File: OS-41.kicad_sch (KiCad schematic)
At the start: 65 parts, among them J1 Conn_02x03_Counter_Clockwise, J2 Conn_01x02_Pin, J3 Conn_01x02_Pin, J4 Conn_Coaxial, SW4 SW_Push, U1 BME280, U2 SI4432-B1-FMR, U3 MCP1640x-xCHY, U4 ATGM336H-5N31, U7 STM32F103C8Tx, Y1 32.768KHz 12.5pF, Y2 8MHz 12pF, Y3 30MHz 10pF

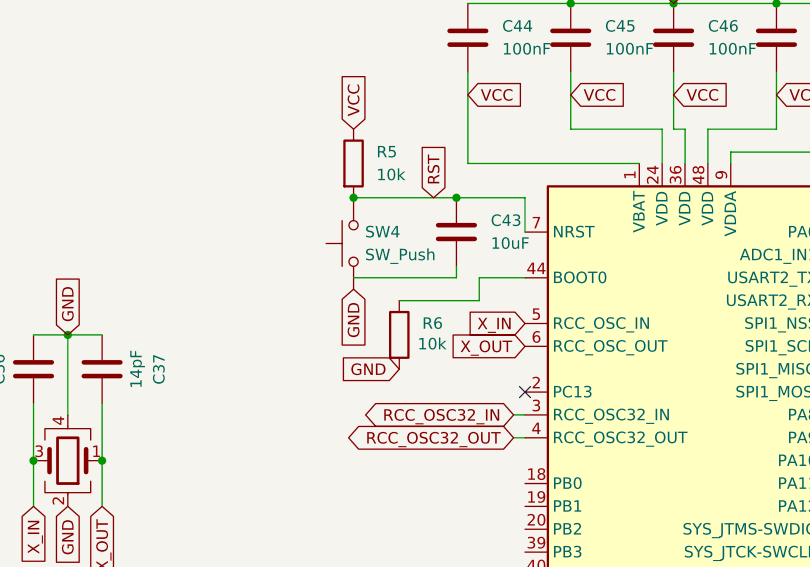
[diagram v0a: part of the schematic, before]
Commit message: Start routing!
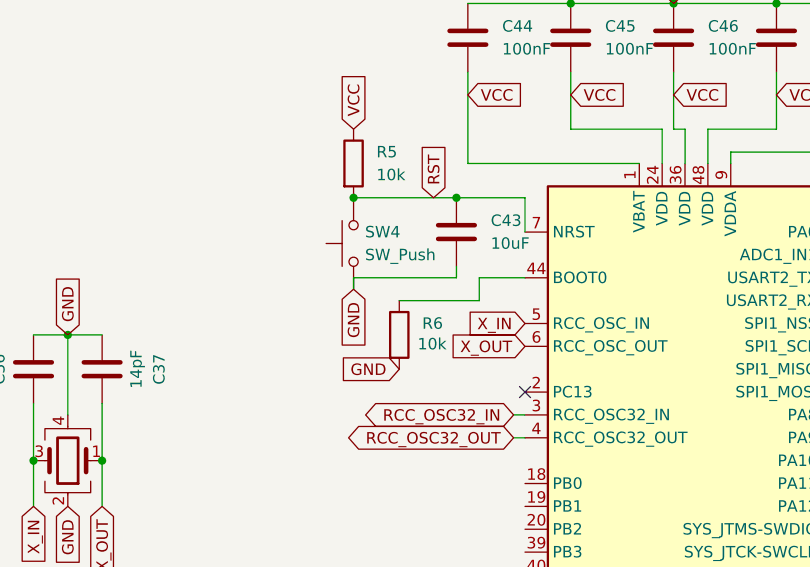
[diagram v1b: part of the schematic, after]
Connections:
- net GND: now also C43.2
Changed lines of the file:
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@@
+	(wire
+		(pts
+			(xy 283.21 60.96) (xy 271.78 60.96)
+		)
+		(stroke
+			(width 0)
+			(type default)
+		)
+	)
 	(wire
 		(pts
@@
 	(wire
 		(pts
-			(xy 271.78 60.96) (xy 283.21 60.96)
-		)
-		(stroke
-			(width 0)
-			(type default)
-		)
-	)
-	(wire
-		(pts
 			(xy 62.23 179.07) (xy 62.23 180.34)
 		)
@@
 		)
 		(stroke
+			(width 0)
+			(type default)
+		)
+	)
+	(wire
+		(pts
+			(xy 271.78 60.96) (xy 271.78 62.23)
+		)
+		(stroke
